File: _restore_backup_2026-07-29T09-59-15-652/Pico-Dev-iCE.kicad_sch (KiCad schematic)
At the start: 110 parts, among them J11 Conn_01x20_Socket, J12 Conn_01x20_Socket, J2 S11, J4 S21, J5 AWG_OUT, J6 PMOD, Q1 2N7002, Q2 2N7002, U1 74LVC1G3157GW, U2 TPH2501-TR, U3 TPH2501-TR, U4 MS9280, U5 MS9708, U6 74LVC1G3157GW, U7 ICE40UP5K-SG48ITR

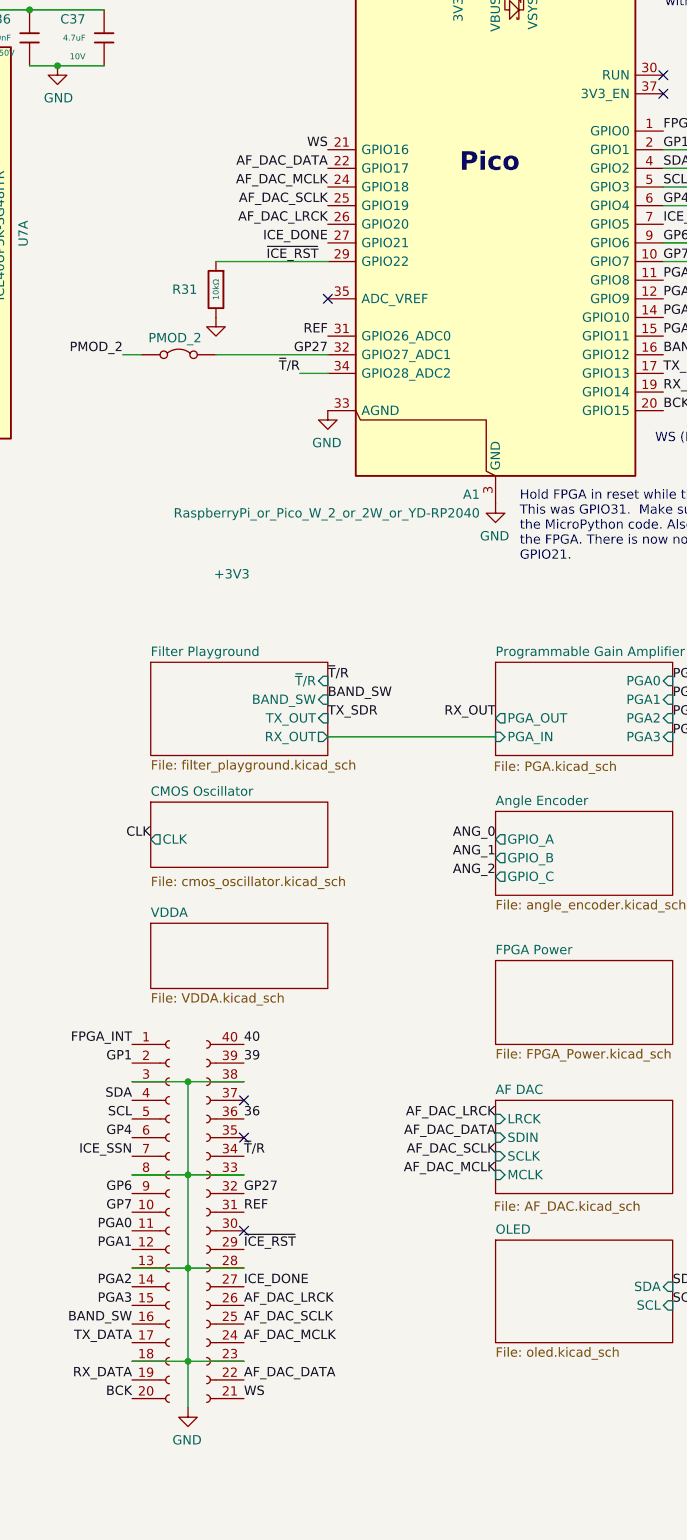
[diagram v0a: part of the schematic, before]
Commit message: Getting ready to submit to JLCPCB.
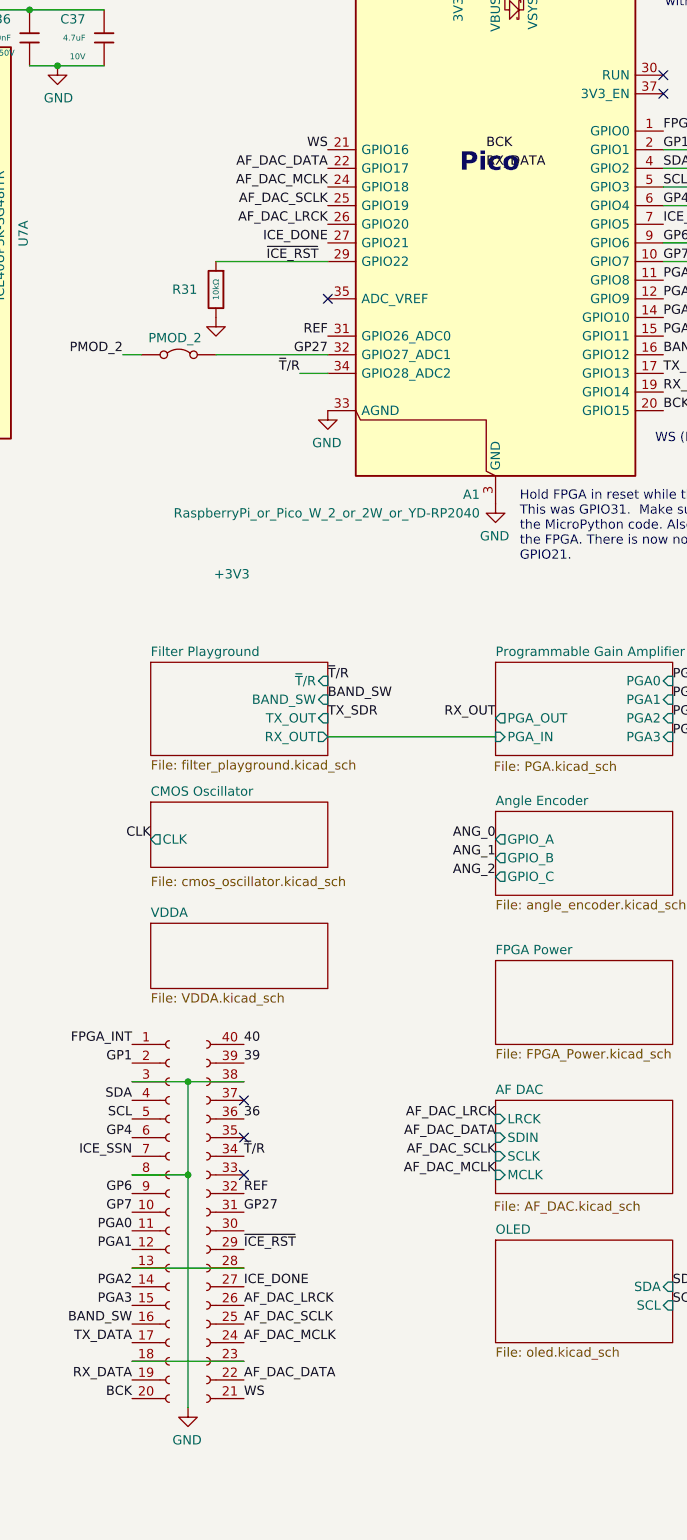
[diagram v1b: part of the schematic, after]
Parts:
- J6: JLCPCB Rotation Offset (none) -> 90
- U7: JLCPCB Rotation Offset (none) -> -90
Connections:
- net GND: no longer J11.13 (Pin_13), J11.18 (Pin_18), J12.23 (Pin_18), J12.28 (Pin_13), J12.33 (Pin_8)
- net GP27: now also J12.31 (Pin_10); no longer J12.32 (Pin_9)
- net REF: now also J12.32 (Pin_9); no longer J12.31 (Pin_10)
- new net: J11.13 (Pin_13), J12.28 (Pin_13)
- new net: J11.18 (Pin_18), J12.23 (Pin_18)
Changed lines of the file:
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@@
 	)
 	(junction
-		(at 322.58 223.52)
-		(diameter 0)
-		(color 0 0 0 0)
-	)
-	(junction
 		(at 208.28 232.41)
 		(diameter 0)
@@
 	)
 	(junction
-		(at 322.58 210.82)
-		(diameter 0)
-		(color 0 0 0 0)
-	)
-	(junction
 		(at 35.56 119.38)
 		(diameter 0)
@@
 	)
 	(no_connect
-		(at 330.2 205.74)
-	)
-	(no_connect
 		(at 48.26 213.36)
 	)
@@
 	)
 	(no_connect
+		(at 330.2 198.12)
+	)
+	(no_connect
 		(at 40.64 213.36)
 	)
@@
 	(wire
 		(pts
-			(xy 314.96 210.82) (xy 322.58 210.82)
+			(xy 314.96 210.82) (xy 330.2 210.82)
 		)
 		(stroke
@@
 	(wire
 		(pts
-			(xy 322.58 210.82) (xy 322.58 223.52)
-		)
-		(stroke
-			(width 0)
-			(type default)
-		)
-	)
-	(wire
-		(pts
 			(xy 402.59 71.12) (xy 405.13 71.12)
 		)
@@
 	(wire
 		(pts
-			(xy 322.58 198.12) (xy 330.2 198.12)
-		)
-		(stroke
-			(width 0)
-			(type default)
-		)
-	)
-	(wire
-		(pts
 			(xy 38.1 195.58) (xy 39.37 195.58)
 		)
@@
 	(wire
 		(pts
-			(xy 322.58 223.52) (xy 330.2 223.52)
-		)
-		(stroke
-			(width 0)
-			(type default)
-		)
-	)
-	(wire
-		(pts
 			(xy 280.67 95.25) (xy 264.16 95.25)
 		)
@@
 	(wire
 		(pts
-			(xy 322.58 210.82) (xy 330.2 210.82)
-		)
-		(stroke
-			(width 0)
-			(type default)
-		)
-	)
-	(wire
-		(pts
 			(xy 74.93 55.88) (xy 74.93 60.96)
 		)
@@
 	(wire
 		(pts
-			(xy 314.96 223.52) (xy 322.58 223.52)
+			(xy 314.96 223.52) (xy 330.2 223.52)
 		)
 		(stroke
@@
 	(wire
 		(pts
-			(xy 322.58 223.52) (xy 322.58 229.87)
-		)
-		(stroke
-			(width 0)
-			(type default)
-		)
-	)
-	(wire
-		(pts
 			(xy 215.9 242.57) (xy 208.28 242.57)
 		)
@@
 	(wire
 		(pts
-			(xy 322.58 198.12) (xy 322.58 210.82)
+			(xy 322.58 198.12) (xy 322.58 229.87)
 		)
 		(stroke
@@
 	)
 	(label "GP27"
-		(at 330.2 200.66 0)
+		(at 330.2 203.2 0)
 		(effects
 			(font
@@
 		)
 	)
+	(label "REF"
+		(at 341.63 83.82 180)
+		(effects
+			(font
+				(size 1.27 1.27)
+				(thickness 0.1588)
+			)
+			(justify right bottom)
+		)
+	)
 	(label "PGA3"
 		(at 388.62 138.43 0)
@@
 		)
 	)
-	(label "REF"
-		(at 341.63 83.82 180)
-		(effects
-			(font
-				(size 1.27 1.27)
-			)
-			(justify right bottom)
-		)
-	)
 	(label "WS"
 		(at 330.2 228.6 0)
@@
 		)
 	)
+	(label "BCK"
+		(at 363.22 58.42 0)
+		(effects
+			(font
+				(size 1.27 1.27)
+			)
+			(justify left bottom)
+		)
+	)
 	(label "~{T}{slash}R"
 		(at 330.2 195.58 0)
@@
 	)
 	(label "REF"
-		(at 330.2 203.2 0)
+		(at 330.2 200.66 0)
 		(effects
 			(font
@@
 		)
 	)
+	(label "RX_DATA"
+		(at 363.22 60.96 0)
+		(effects
+			(font
+				(size 1.27 1.27)
+			)
+			(justify left bottom)
+		)
+	)
 	(label "SCL"
 		(at 388.62 215.9 0)
@@
 			)
 		)
-		(property "JLCPCB Rotation Offset" ""
-			(at 45.72 223.52 90)
-			(hide yes)
-			(show_name no)
-			(do_not_autoplace no)
-			(effects
-				(font
-					(size 1.27 1.27)
-				)
-			)
-		)
 		(pin "2"
 		)
@@
 			)
 		)
-		(property "JLCPCB Rotation Offset" ""
-			(at 320.04 203.2 0)
-			(hide yes)
-			(show_name no)
-			(do_not_autoplace no)
-			(effects
-				(font
-					(size 1.27 1.27)
-				)
-			)
-		)
 		(pin "17"
 		)
@@
 			)
 		)
-		(property "JLCPCB Rotation Offset" ""
-			(at 40.64 87.63 90)
-			(hide yes)
-			(show_name no)
-			(do_not_autoplace no)
-			(effects
-				(font
-					(size 1.27 1.27)
-				)
-			)
-		)
 		(pin "2"
 		)
@@
 			)
 		)
-		(property "JLCPCB Rotation Offset" ""
-			(at 59.69 58.42 0)
-			(hide yes)
-			(show_name no)
-			(do_not_autoplace no)
-			(effects
-				(font
-					(size 1.27 1.27)
-				)
-			)
-		)
 		(pin "2"
 		)
@@
 			)
 		)
-		(property "JLCPCB Rotation Offset" ""
+		(property "JLCPCB Rotation Offset" "-90"
 			(at 189.23 66.04 90)
 			(hide yes)
@@
 			)
 		)
-		(property "JLCPCB Rotation Offset" ""
+		(property "JLCPCB Rotation Offset" "90"
 			(at 238.76 88.9 0)
 			(hide yes)
@@
 			)
 		)
-		(property "JLCPCB Rotation Offset" ""
-			(at 41.91 190.5 90)
-			(hide yes)
-			(show_name no)
-			(do_not_autoplace no)
-			(effects
-				(font
-					(size 1.27 1.27)
-				)
-			)
-		)
 		(pin "4"
 		)
@@
 			)
 		)
-		(property "JLCPCB Rotation Offset" ""
+		(property "JLCPCB Rotation Offset" "-90"
 			(at 238.76 59.69 90)
 			(hide yes)
@@
 			)
 		)
-		(property "JLCPCB Rotation Offset" ""
+		(property "JLCPCB Rotation Offset" "-90"
 			(at 290.83 69.85 90)
 			(hide yes)
@@
 			(hide yes)
 			(show_name no)
-			(do_not_autoplace no)
-			(effects
-				(font
-					(size 1.27 1.27)
-				)
-			)
-		)
-		(property "JLCPCB Rotation Offset" ""
-			(at 97.79 193.04 90)
-			(hide yes)
-			(show_name no)
